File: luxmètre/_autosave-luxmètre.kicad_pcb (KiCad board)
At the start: 2 copper layers, 91.4 x 86.4 mm, 84 parts, among them J1 USB_A, J2 Conn_01x08, J3 Conn_01x01, J4 Conn_01x04, J5 Conn_01x01, J6 Conn_01x01, J7 Conn_01x03, J8 Conn_01x03, SW1 B3S-1000P, U1 ESP32-WROOM-32, U10 MAX1674EUA+T, U11 MCP73831-2-MC, U3 ADC-10-4+, U4 RF-LORA-868-SO, U5 PCA9537DP, U6 FT232HL, U7 ILB1206ER260V, U8 ILB1206ER260V, U9 ILB1206ER260V, Y1 12MHz

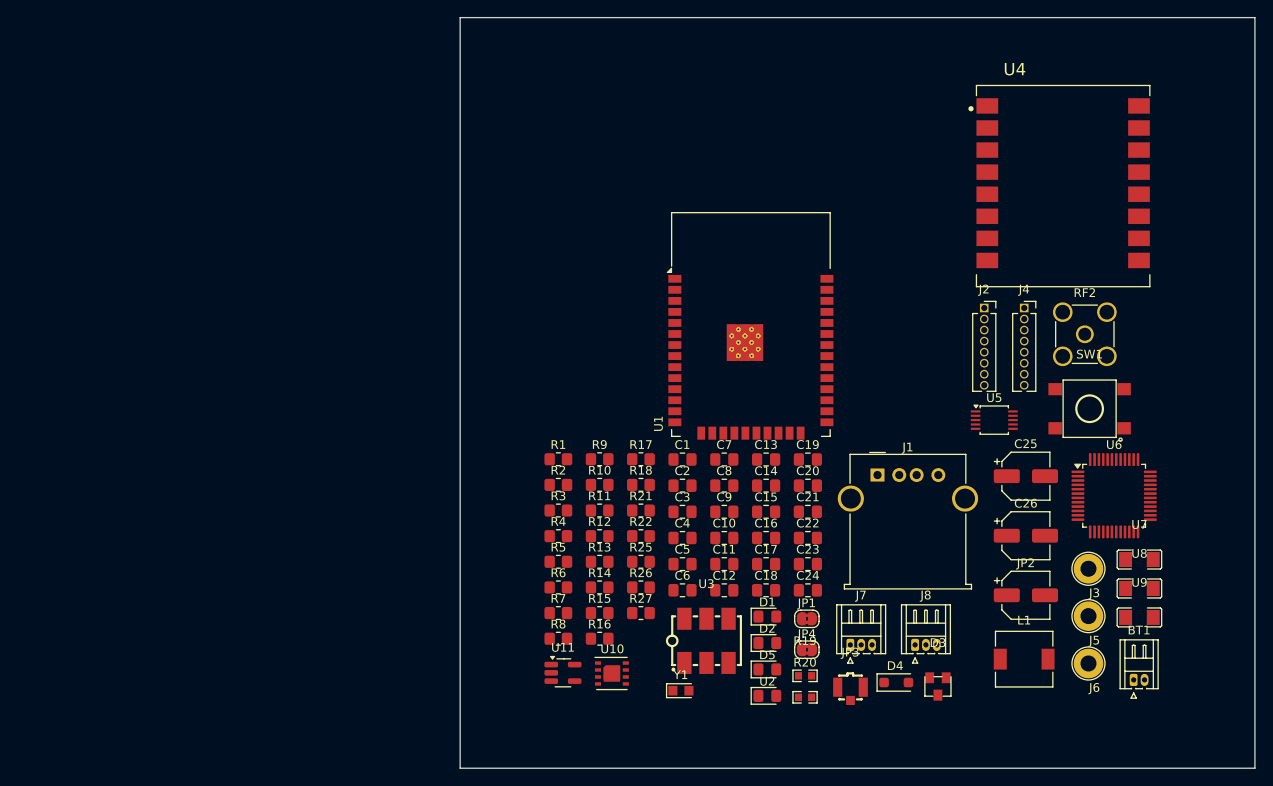
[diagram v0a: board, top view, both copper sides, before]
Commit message: routage computing unit bloc
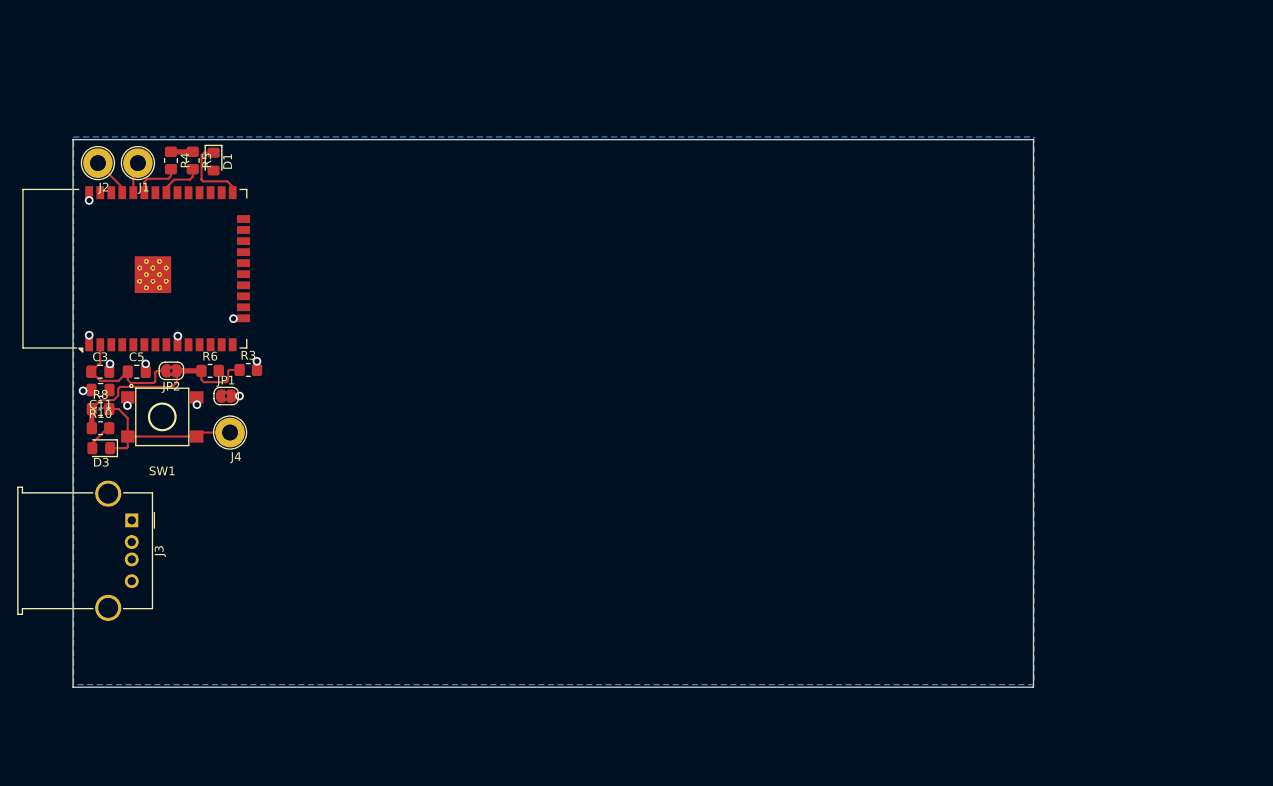
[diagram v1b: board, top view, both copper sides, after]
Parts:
- removed BT1: Battery, Connector_Hirose:Hirose_DF13-02P-1.25DS_1x02_P1.25mm_Horizontal
- removed C1, C10, C13, C14, C15, C16, C2, C23, C24, C7, C8, C9: 100nF, Capacitor_SMD:C_0805_2012Metric_Pad1.18x1.45mm_HandSolder
- removed C12: 3.3uF, Capacitor_SMD:C_0805_2012Metric_Pad1.18x1.45mm_HandSolder
- removed C17, C18, C22, C4, C6: 10uF, Capacitor_SMD:C_0805_2012Metric_Pad1.18x1.45mm_HandSolder
- removed C19, C20, C21: 10nF, Capacitor_SMD:C_0805_2012Metric_Pad1.18x1.45mm_HandSolder
- removed C25, C26: 47uF, Capacitor_SMD:CP_Elec_5x5.4
- removed D2, D5: LED, LED_SMD:LED_0805_2012Metric_Pad1.15x1.40mm_HandSolder
- removed D4: MBR0520LT, Diode_SMD:D_SOD-123F
- removed J5, J6: Conn_01x01, TestPoint:TestPoint_Loop_D2.50mm_Drill1.85mm
- removed J7, J8: Conn_01x03, Connector_Hirose:Hirose_DF13-03P-1.25DS_1x03_P1.25mm_Horizontal
- removed JP3: U.FL-R-SMT-1(80), easyeda2kicad:RF-SMD_FRF05002-JSS103M
- removed JP4: Jumper_2_Open, Jumper:SolderJumper-2_P1.3mm_Bridged2Bar_RoundedPad1.0x1.5mm
- removed L1: 22uH, Inductor_SMD:L_6.3x6.3_H3
- removed R1, R22, R25: 100k, Resistor_SMD:R_0805_2012Metric_Pad1.20x1.40mm_HandSolder
- removed R11, R7: 270R, Resistor_SMD:R_0805_2012Metric_Pad1.20x1.40mm_HandSolder
- removed R12, R9: 68R, Resistor_SMD:R_0805_2012Metric_Pad1.20x1.40mm_HandSolder
- removed R13, R17, R18: 10k, Resistor_SMD:R_0805_2012Metric_Pad1.20x1.40mm_HandSolder
- removed R14, R15: 470R, Resistor_SMD:R_0805_2012Metric_Pad1.20x1.40mm_HandSolder
- removed R16: 47k, Resistor_SMD:R_0805_2012Metric_Pad1.20x1.40mm_HandSolder
- removed R19, R20: V5.5MLA0603NH, easyeda2kicad:R0603
- removed R2: 4k7, Resistor_SMD:R_0805_2012Metric_Pad1.20x1.40mm_HandSolder
- removed R21: 113k, Resistor_SMD:R_0805_2012Metric_Pad1.20x1.40mm_HandSolder
- removed R26: 1.5k, Resistor_SMD:R_0805_2012Metric_Pad1.20x1.40mm_HandSolder
- removed R27: 2k, Resistor_SMD:R_0805_2012Metric_Pad1.20x1.40mm_HandSolder
- removed RF2: HJ-SMA313, Connector_Coaxial:SMA_Amphenol_901-144_Vertical
- removed U1: ESP32-WROOM-32, RF_Module:ESP32-WROOM-32
- removed U10: MAX1674EUA+T, Converter_DCDC:Converter_DCDC_Cyntec_MUN12AD01-SH
- removed U11: MCP73831-2-MC, Package_TO_SOT_SMD:SOT-23-5_HandSoldering
- removed U2: ~, LED_SMD:LED_0805_2012Metric_Pad1.15x1.40mm_HandSolder
- removed U3: ADC-10-4+, My_symbols:XFMR-SMD_6P-L7.9-W5.6-P2.54-LS7.0-BL
- removed U5: PCA9537DP, Package_SO:TSSOP-10_3x3mm_P0.5mm
- removed U6: FT232HL, Package_QFP:LQFP-48_7x7mm_P0.5mm
- removed U7, U8, U9: ILB1206ER260V, easyeda2kicad:L1206
- removed Y1: 12MHz, Crystal:Crystal_SMD_2012-2Pin_2.0x1.2mm_HandSoldering
- C5: value 100nF -> 10uF
- D3: value PGB102ST23WR -> LED; footprint easyeda2kicad:SOT-23_L3.0-W2.2-P0.95-LS2.2-TR -> LED_SMD:LED_0805_2012Metric_Pad1.15x1.40mm_HandSolder
- J1: value USB_A -> Conn_01x01; footprint Connector_USB:USB_A_Molex_67643_Horizontal -> TestPoint:TestPoint_Loop_D2.50mm_Drill1.85mm
- J2: value Conn_01x08 -> Conn_01x01; footprint Connector_PinSocket_1.27mm:PinSocket_1x08_P1.27mm_Vertical -> TestPoint:TestPoint_Loop_D2.50mm_Drill1.85mm
- J3: value Conn_01x01 -> USB_A; footprint TestPoint:TestPoint_Loop_D2.50mm_Drill1.85mm -> Connector_USB:USB_A_Molex_67643_Horizontal
- J4: value Conn_01x04 -> Conn_01x01; footprint Connector_PinSocket_1.27mm:PinSocket_1x08_P1.27mm_Vertical -> TestPoint:TestPoint_Loop_D2.50mm_Drill1.85mm
- JP2: footprint Capacitor_SMD:CP_Elec_5x5.4 -> Jumper:SolderJumper-2_P1.3mm_Bridged2Bar_RoundedPad1.0x1.5mm
- R10: value 68R -> 470R
- R3: value 4k7 -> 10k
- R4: value 10k -> 4k7
- R5: value 100k -> 4k7
- R6: value R -> 470R
- R8: value 68R -> 10k
- U4: value RF-LORA-868-SO -> ESP32-WROOM-32; footprint My_symbols:XCVR_RF-LORA-868-SO -> RF_Module:ESP32-WROOM-32
- moved J3 110.2 mm to (56.2, 93.4), turned to -90 degrees
- moved SW1 106.7 mm to (59.7, 81.5), turned to 180 degrees
- moved U4 104.2 mm to (59.5, 64.5), turned to 90 degrees
- moved J2 103.3 mm to (52.3, 52.3)
- moved JP2 101.6 mm to (60.8, 76.2), turned to 180 degrees
- moved D3 100.1 mm to (52.7, 85.1), turned to 180 degrees
- moved J4 92.5 mm to (67.5, 83.3)
- moved J1 92.3 mm to (56.9, 52.3)
- moved D1 82.5 mm to (65.6, 52.1), turned to -90 degrees
- moved C11 74.5 mm to (52.6, 78.4), turned to 180 degrees
- moved JP1 71.6 mm to (67.1, 79.1)
- moved C3 68.9 mm to (52.6, 76.3)
- moved C5 66.6 mm to (56.8, 76.3)
- moved R5 62.5 mm to (63.2, 52.0), turned to -90 degrees
- moved R4 62.1 mm to (60.7, 52.0), turned to -90 degrees
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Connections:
- C11 pad 1: Net-(U6-VCCA) -> /RST
- C3 pad 1: +3.3V -> Net-(JP2-B)
- C5 pad 1: Net-(JP4-B) -> Net-(JP2-B)
- D1 pad 1: //RST -> /BOOT
- D3 pad 1: /dp -> /RST
- D3 pad 2: /dm -> Net-(D3-A)
- J1 pad 1: /5V_usb -> /RXD
- J2 pad 1: /DIO0 -> /TXD
- J3 pad 1: //RST -> /5V_usb
- J4 pad 1: /RST_L -> /RST
- R10 pad 1: GND -> +3.3V
- R10 pad 2: Net-(R10-Pad2) -> Net-(D3-A)
- R3 pad 2: /SCL -> GND
- R4 pad 2: GND -> /SCL
- R5 pad 1: GND -> +3.3V
- R5 pad 2: /TX_SW -> /SDA
- R6 pad 1: GND -> +3.3V
- R6 pad 2: Net-(U3-TERM) -> Net-(D1-A)
- R8 pad 1: GND -> +3.3V
- R8 pad 2: /C -> /RST
- SW1 pad 3: //RST -> /RST
- SW1 pad 4: //RST -> /RST
- U4 pad 1: /ANT -> GND
- U4 pad 10: /DIO4 -> unconnected-(U4-IO25-Pad10)
- U4 pad 11: /DIO3 -> unconnected-(U4-IO26-Pad11)
- U4 pad 12: /RST_L -> unconnected-(U4-IO27-Pad12)
- U4 pad 14: /MOSI_L -> /MISO_L
- U4 pad 15: /MISO_L -> GND
- U4 pad 16: //SEL -> /MOSI_L
- U4 pad 2: GND -> Net-(JP2-B)
- U4 pad 3: Net-(JP2-B) -> /RST
- U4 pad 4: /RX_SW -> unconnected-(U4-SENSOR_VP-Pad4)
- U4 pad 5: /TX_SW -> unconnected-(U4-SENSOR_VN-Pad5)
- U4 pad 6: /DIO0 -> unconnected-(U4-IO34-Pad6)
- U4 pad 7: /DIO1 -> unconnected-(U4-IO35-Pad7)
- U4 pad 8: /DIO2 -> unconnected-(U4-IO32-Pad8)
- U4 pad 9: /DIO5 -> GND
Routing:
- net +3.3V: track 0.00 -> 27.1 mm
- net /RST: track 0.00 -> 19.9 mm
- net Net-(JP2-B): track 0.00 -> 15.2 mm
- net GND: track 0.00 -> 10.8 mm, vias 0 -> 11
- net /BOOT: track 0.00 -> 8.95 mm
- net /SCL: track 0.00 -> 5.37 mm
- net /SDA: track 0.00 -> 5.01 mm
- net /TXD: track 0.00 -> 4.56 mm
- net /RXD: track 0.00 -> 3.62 mm
- net Net-(D3-A): track 0.00 -> 3.23 mm
- added copper zone on B.Cu, net GND
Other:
- board size 91.4 x 86.4 mm -> 110.5 x 63 mm
- copper layers 2 -> 4

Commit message: pcb
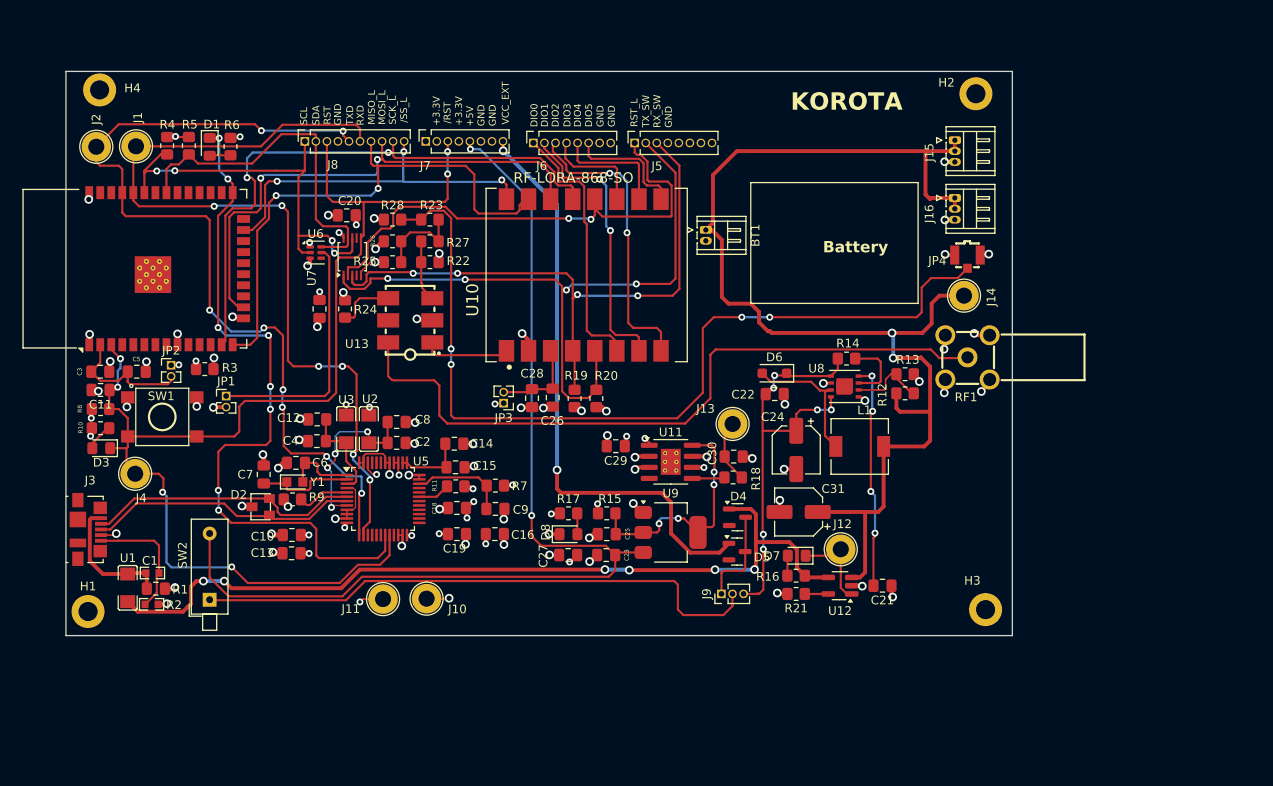
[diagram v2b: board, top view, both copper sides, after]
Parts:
- added BT1: Battery, Connector_Hirose:Hirose_DF13-02P-1.25DS_1x02_P1.25mm_Horizontal, F.Cu at (122.2, 60.0)
- added C1: 10uF, Capacitor_SMD:C_0805_2012Metric_Pad1.18x1.45mm_HandSolder, F.Cu at (59.0, 101.3)
- added C10: 100nF, Capacitor_SMD:C_0805_2012Metric_Pad1.18x1.45mm_HandSolder, F.Cu at (74.6, 95.1)
- added C12: 100nF, Capacitor_SMD:C_0805_2012Metric_Pad1.18x1.45mm_HandSolder, F.Cu at (77.5, 81.8)
- added C13: 100nF, Capacitor_SMD:C_0805_2012Metric_Pad1.18x1.45mm_HandSolder, F.Cu at (74.6, 97.2)
- added C14: 3.3uF, Capacitor_SMD:C_0805_2012Metric_Pad1.18x1.45mm_HandSolder, F.Cu at (93.3, 84.6)
- added C15: 100nF, Capacitor_SMD:C_0805_2012Metric_Pad1.18x1.45mm_HandSolder, F.Cu at (93.4, 87.3)
- added C16: 100nF, Capacitor_SMD:C_0805_2012Metric_Pad1.18x1.45mm_HandSolder, F.Cu at (98.0, 95.0)
- added C17: 100nF, Capacitor_SMD:C_0805_2012Metric_Pad1.18x1.45mm_HandSolder, F.Cu at (77.8, 69.1)
- added C18: 100nF, Capacitor_SMD:C_0805_2012Metric_Pad1.18x1.45mm_HandSolder, F.Cu at (93.6, 92.0)
- added C19: 100nF, Capacitor_SMD:C_0805_2012Metric_Pad1.18x1.45mm_HandSolder, F.Cu at (93.6, 95.0)
- added C2: 10uF, Capacitor_SMD:C_0805_2012Metric_Pad1.18x1.45mm_HandSolder, F.Cu at (86.7, 84.5)
- added C20: 100nF, Capacitor_SMD:C_0805_2012Metric_Pad1.18x1.45mm_HandSolder, F.Cu at (80.9, 58.3)
- added C21: 100nF, Capacitor_SMD:C_0805_2012Metric_Pad1.18x1.45mm_HandSolder, F.Cu at (142.6, 100.9)
- added C22: 100nF, Capacitor_SMD:C_0805_2012Metric_Pad1.18x1.45mm_HandSolder, F.Cu at (130.2, 78.9)
- added C23: 10uF, Capacitor_SMD:C_0805_2012Metric_Pad1.18x1.45mm_HandSolder, F.Cu at (110.8, 97.4)
- added C24: 47uF, Capacitor_SMD:CP_Elec_5x5.4, F.Cu at (132.7, 85.3)
- added C25: 10uF, Capacitor_SMD:C_0805_2012Metric_Pad1.18x1.45mm_HandSolder, F.Cu at (110.8, 95.0)
- added C26: 100nF, Capacitor_SMD:C_0805_2012Metric_Pad1.18x1.45mm_HandSolder, F.Cu at (104.6, 79.3)
- added C27: 100nF, Capacitor_SMD:C_0805_2012Metric_Pad1.18x1.45mm_HandSolder, F.Cu at (106.4, 97.4)
- added C28: 10uF, Capacitor_SMD:C_0805_2012Metric_Pad1.18x1.45mm_HandSolder, F.Cu at (102.2, 79.3)
- added C29: 100nF, Capacitor_SMD:C_0805_2012Metric_Pad1.18x1.45mm_HandSolder, F.Cu at (111.9, 84.9)
- added C30: 10nF, Capacitor_SMD:C_0805_2012Metric_Pad1.18x1.45mm_HandSolder, F.Cu at (125.4, 86.1)
- added C31: 47uF, Capacitor_SMD:CP_Elec_5x5.4, F.Cu at (132.9, 92.4)
- added C4: 10uF, Capacitor_SMD:C_0805_2012Metric_Pad1.18x1.45mm_HandSolder, F.Cu at (77.5, 84.3)
- added C6: 10nF, Capacitor_SMD:C_0805_2012Metric_Pad1.18x1.45mm_HandSolder, F.Cu at (75.1, 86.8)
- added C7: 10nF, Capacitor_SMD:C_0805_2012Metric_Pad1.18x1.45mm_HandSolder, F.Cu at (71.4, 88.1)
- added C8: 100nF, Capacitor_SMD:C_0805_2012Metric_Pad1.18x1.45mm_HandSolder, F.Cu at (86.7, 82.1)
- added C9: 10nF, Capacitor_SMD:C_0805_2012Metric_Pad1.18x1.45mm_HandSolder, F.Cu at (98.0, 92.1)
- added D2: PGB102ST23WR, easyeda2kicad:SOT-23_L3.0-W2.2-P0.95-LS2.2-TR, F.Cu at (71.0, 91.8)
- added D4: BAT54C, Package_TO_SOT_SMD:SOT-23, F.Cu at (125.9, 93.0)
- added D5: BAT54C, Package_TO_SOT_SMD:SOT-23, F.Cu at (125.8, 97.0)
- added D6: MBR0520LT, Diode_SMD:D_SOD-123F, F.Cu at (130.1, 76.5)
- added D7: LED, LED_SMD:LED_0805_2012Metric_Pad1.15x1.40mm_HandSolder, F.Cu at (132.7, 97.5)
- added D8: LED, LED_SMD:LED_0805_2012Metric_Pad1.15x1.40mm_HandSolder, F.Cu at (106.4, 95.0)
- added H1: MountingHole, MountingHole:MountingHole_2.2mm_M2_DIN965_Pad, F.Cu at (51.2, 103.9)
- added H2: MountingHole, MountingHole:MountingHole_2.2mm_M2_DIN965_Pad, F.Cu at (153.3, 44.3)
- added H3: MountingHole, MountingHole:MountingHole_2.2mm_M2_DIN965_Pad, F.Cu at (154.4, 103.7)
- added H4: MountingHole, MountingHole:MountingHole_2.2mm_M2_DIN965_Pad, F.Cu at (52.5, 43.9)
- added J10: Conn_01x01, TestPoint:TestPoint_Loop_D2.50mm_Drill1.85mm, F.Cu at (90.1, 102.4)
- added J11: Conn_01x01, TestPoint:TestPoint_Loop_D2.50mm_Drill1.85mm, F.Cu at (85.1, 102.5)
- added J12: Conn_01x01, TestPoint:TestPoint_Loop_D2.50mm_Drill1.85mm, F.Cu at (137.8, 96.7)
- added J13: Conn_01x01, TestPoint:TestPoint_Loop_D2.50mm_Drill1.85mm, F.Cu at (125.3, 82.3)
- added J14: Conn_01x01, TestPoint:TestPoint_Loop_D2.50mm_Drill1.85mm, F.Cu at (151.9, 67.5)
- added J15: Conn_01x03, Connector_Hirose:Hirose_DF13-03P-1.25DS_1x03_P1.25mm_Horizontal, F.Cu at (150.9, 49.7)
- added J16: Conn_01x03, Connector_Hirose:Hirose_DF13-03P-1.25DS_1x03_P1.25mm_Horizontal, F.Cu at (150.9, 56.3)
- added J5: Conn_01x04, Connector_PinSocket_1.27mm:PinSocket_1x08_P1.27mm_Vertical, F.Cu at (114.1, 50.0)
- added J6: Conn_01x08, Connector_PinSocket_1.27mm:PinSocket_1x08_P1.27mm_Vertical, F.Cu at (102.4, 50.0)
- added J7: Conn_01x08, Connector_PinSocket_1.27mm:PinSocket_1x08_P1.27mm_Vertical, F.Cu at (90.0, 49.8)
- added J8: Conn_01x10, Connector_PinSocket_1.27mm:PinSocket_1x10_P1.27mm_Vertical, F.Cu at (76.1, 49.8)
- added J9: Conn_01x03, Connector_PinHeader_1.27mm:PinHeader_1x03_P1.27mm_Vertical, F.Cu at (124.0, 101.9)
- added JP3: Jumper_2_Open, Connector_PinHeader_1.27mm:PinHeader_1x02_P1.27mm_Vertical, F.Cu at (99.0, 79.9)
- added JP4: U.FL-R-SMT-1(80), easyeda2kicad:RF-SMD_FRF05002-JSS103M, F.Cu at (152.3, 63.6)
- added L1: 22uH, Inductor_SMD:L_6.3x6.3_H3, F.Cu at (139.9, 84.9)
- added R1: V5.5MLA0603NH, easyeda2kicad:R0603, F.Cu at (58.6, 99.5)
- added R11: 47k, Resistor_SMD:R_0805_2012Metric_Pad1.20x1.40mm_HandSolder, F.Cu at (93.5, 89.5)
- added R12: 113k, Resistor_SMD:R_0805_2012Metric_Pad1.20x1.40mm_HandSolder, F.Cu at (145.2, 78.8)
- added R13: 100k, Resistor_SMD:R_0805_2012Metric_Pad1.20x1.40mm_HandSolder, F.Cu at (145.2, 76.6)
- added R14: 100k, Resistor_SMD:R_0805_2012Metric_Pad1.20x1.40mm_HandSolder, F.Cu at (138.4, 74.8)
- added R15: 0R1, Resistor_SMD:R_0805_2012Metric_Pad1.20x1.40mm_HandSolder, F.Cu at (110.8, 92.6)
- added R16: 1.5k, Resistor_SMD:R_0805_2012Metric_Pad1.20x1.40mm_HandSolder, F.Cu at (132.6, 99.8)
- added R17: 330R, Resistor_SMD:R_0805_2012Metric_Pad1.20x1.40mm_HandSolder, F.Cu at (106.4, 92.6)
- added R18: 330R, Resistor_SMD:R_0805_2012Metric_Pad1.20x1.40mm_HandSolder, F.Cu at (125.4, 88.5)
- added R19: 100k, Resistor_SMD:R_0805_2012Metric_Pad1.20x1.40mm_HandSolder, F.Cu at (107.2, 79.4)
- added R2: V5.5MLA0603NH, easyeda2kicad:R0603, F.Cu at (58.5, 103.1)
- added R20: 100k, Resistor_SMD:R_0805_2012Metric_Pad1.20x1.40mm_HandSolder, F.Cu at (109.7, 79.4)
- added R21: 2k, Resistor_SMD:R_0805_2012Metric_Pad1.20x1.40mm_HandSolder, F.Cu at (132.6, 101.9)
- added R22: 68R, Resistor_SMD:R_0805_2012Metric_Pad1.20x1.40mm_HandSolder, F.Cu at (90.5, 63.7)
- added R23: 270R, Resistor_SMD:R_0805_2012Metric_Pad1.20x1.40mm_HandSolder, F.Cu at (90.5, 61.3)
- added R24: R, Resistor_SMD:R_0805_2012Metric_Pad1.20x1.40mm_HandSolder, F.Cu at (80.7, 69.1)
- added R25: 68R, Resistor_SMD:R_0805_2012Metric_Pad1.20x1.40mm_HandSolder, F.Cu at (86.2, 63.7)
- added R26: 68R, Resistor_SMD:R_0805_2012Metric_Pad1.20x1.40mm_HandSolder, F.Cu at (86.2, 61.3)
- added R27: 270R, Resistor_SMD:R_0805_2012Metric_Pad1.20x1.40mm_HandSolder, F.Cu at (90.5, 58.8)
- added R28: 68R, Resistor_SMD:R_0805_2012Metric_Pad1.20x1.40mm_HandSolder, F.Cu at (86.2, 58.8)
- added R7: 10k, Resistor_SMD:R_0805_2012Metric_Pad1.20x1.40mm_HandSolder, F.Cu at (98.0, 89.4)
- added R9: 10k, Resistor_SMD:R_0805_2012Metric_Pad1.20x1.40mm_HandSolder, F.Cu at (74.7, 91.0)
- added RF1: HJ-SMA313, easyeda2kicad:SMA-TH_HJ-2LC15SF048, F.Cu at (152.3, 74.7)
- added SW2: SW_DIP_x01, Button_Switch_THT:SW_DIP_SPSTx01_Piano_10.8x4.1mm_W7.62mm_P2.54mm, F.Cu at (65.2, 102.5)
- added U1: ILB1206ER260V, easyeda2kicad:L1206, F.Cu at (55.7, 101.2)
- added U10: RF-LORA-868-SO, My_symbols:XCVR_RF-LORA-868-SO, F.Cu at (108.5, 65.2)
- added U11: AD8418, Package_SO:SOIC-8-1EP_3.9x4.9mm_P1.27mm_EP2.29x3mm_ThermalVias, F.Cu at (118.2, 86.7)
- added U12: MCP73831-2-MC, Package_TO_SOT_SMD:SOT-23-5_HandSoldering, F.Cu at (137.7, 100.9)
- added U13: ADC-10-4+, My_symbols:XFMR-SMD_6P-L7.9-W5.6-P2.54-LS7.0-BL, F.Cu at (88.2, 70.4)
- added U2: ILB1206ER260V, easyeda2kicad:L1206, F.Cu at (83.5, 82.9)
- added U3: ILB1206ER260V, easyeda2kicad:L1206, F.Cu at (80.9, 82.9)
- added U5: FT232HL, Package_QFP:LQFP-48_7x7mm_P0.5mm, F.Cu at (85.1, 90.9)
- added U6: ~, OptoDevice:AMS_TSL25911FN, F.Cu at (77.4, 62.6)
- added U7: PCA9537DP, Package_SO:TSSOP-10_3x3mm_P0.5mm, F.Cu at (81.6, 63.1)
- added U8: MAX1674EUA+T, Converter_DCDC:Converter_DCDC_Cyntec_MUN12AD01-SH, F.Cu at (138.2, 78.0)
- added U9: LM1117MP-3.3, Package_TO_SOT_SMD:SOT-223-3_TabPin2, F.Cu at (118.2, 94.8)
- added Y1: 12MHz, Crystal:Crystal_SMD_2012-2Pin_2.0x1.2mm_HandSoldering, F.Cu at (75.0, 89.0)
- J3: footprint Connector_USB:USB_A_Molex_67643_Horizontal -> Connector_USB:USB_Micro-B_Molex_47346-0001
- JP1, JP2: footprint Jumper:SolderJumper-2_P1.3mm_Bridged2Bar_RoundedPad1.0x1.5mm -> Connector_PinHeader_1.27mm:PinHeader_1x02_P1.27mm_Vertical
- moved R6 25.9 mm to (67.6, 50.4), turned to -90 degrees
- moved J4 11.9 mm to (56.6, 88.0)
- moved J3 5.11 mm to (51.2, 94.5)
- moved R3 5.01 mm to (64.6, 76.0)
- moved J1 1.94 mm to (56.7, 50.4)
- moved J2 1.89 mm to (52.1, 50.4)
- moved D1 1.76 mm to (65.2, 50.4)
- moved R4 1.76 mm to (60.3, 50.3)
- moved R5 1.76 mm to (62.8, 50.3)
- moved JP2 0.64 mm to (60.7, 75.6), turned to 0 degrees
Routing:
- net V_BAT: track 0.00 -> 140.2 mm, vias 0 -> 2
- net /RST: track 19.9 -> 143.8 mm, vias 0 -> 6
- net +5V: track 0.00 -> 118.5 mm, vias 0 -> 2
- net Net-(JP4-SIG): track 0.00 -> 101.9 mm, vias 0 -> 4
- net GND: track 10.8 -> 110.7 mm, vias 11 -> 76
- net /TXD: track 4.56 -> 102.2 mm, vias 0 -> 8
- net VCC_USB: track 0.00 -> 97.6 mm, vias 0 -> 6
- net /RXD: track 3.62 -> 98.6 mm, vias 0 -> 6
- net Net-(U13-OUTPUT): track 0.00 -> 81.7 mm
- net /TX_SW: track 0.00 -> 79.3 mm, vias 0 -> 4
- net /BOOT: track 8.95 -> 81.3 mm, vias 0 -> 8
- net /RX_SW: track 0.00 -> 71.2 mm, vias 0 -> 4
- net /SCK_L: track 0.00 -> 67.9 mm, vias 0 -> 2
- net VCC_EXT: track 0.00 -> 67.9 mm, vias 0 -> 2
- net Net-(J9-Pin_2): track 0.00 -> 66.2 mm
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- added copper zone on In2.Cu, net +3.3V
- added copper zone on In1.Cu, net GND
- removed copper zone on B.Cu, net GND
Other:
- board size 110.5 x 63 mm -> 108.9 x 64.9 mm
- board text added: "+3.3V"
- board text added: "+5V"
- board text added: "/RST"
- board text added: "/SS_L"
- board text added: "Battery"
- board text added: "DIO0"
- board text added: "DIO1"
- board text added: "DIO2"
- board text added: "DIO3"
- board text added: "DIO4"
- board text added: "DIO5"
- board text added: "GND"
- board text added: "KOROTA"
- board text added: "MISO_L"
- board text added: "MOSI_L"
- board text added: "RF-LORA-868-SO"
- board text added: "RST"
- board text added: "RST_L"
- board text added: "RXD"
- board text added: "RX_SW"
- board text added: "SCK_L"
- board text added: "SCL"
- board text added: "SDA"
- board text added: "TXD"
- board text added: "TX_SW"
- board text added: "VCC_EXT"

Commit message: pcb
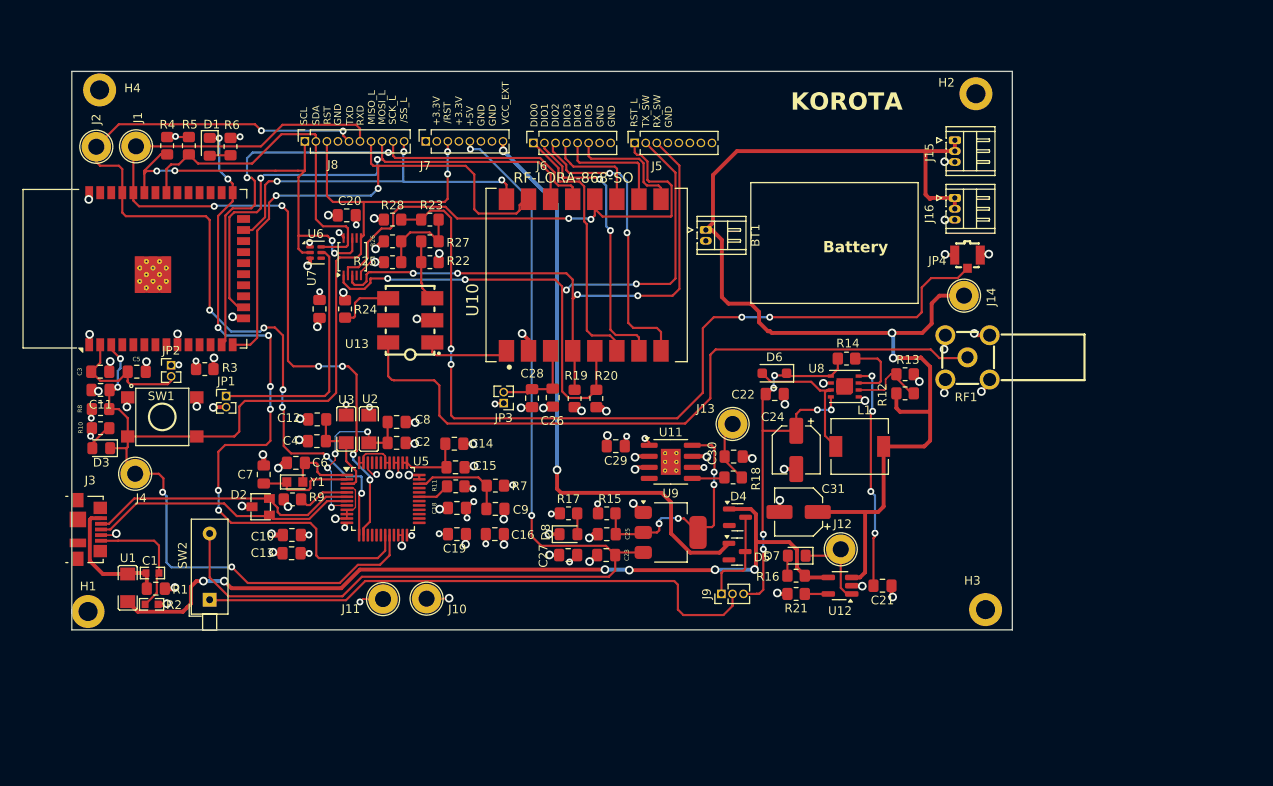
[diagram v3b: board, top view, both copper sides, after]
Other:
- board size 108.9 x 64.9 mm -> 108.2 x 64.2 mm
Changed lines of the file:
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@@
 			(outputformat 1)
 			(mirror no)
-			(drillshape 1)
+			(drillshape 0)
 			(scaleselection 1)
 			(outputdirectory "")
@@
 	)
 	(gr_rect
-		(start 48.63 41.75)
-		(end 157.51 106.66)
+		(start 49.3 41.75)
+		(end 157.51 106)
 		(stroke
 			(width 0.05)
@@
 		(polygon
 			(pts
-				(xy 49.52 42.09) (xy 158.12 41.9) (xy 157.31 106.38) (xy 48.68 106.79)
+				(xy 48.42 41.69) (xy 157.02 41.5) (xy 158.51 105.98) (xy 49.88 106.39)
 			)
 		)
@@
 		(polygon
 			(pts
-				(xy 49.1 42.12) (xy 158.13 41.25) (xy 157.08 106.27) (xy 48.67 107.15)
+				(xy 49 42.12) (xy 158.03 41.25) (xy 157.78 105.67) (xy 49.37 106.55)
 			)
 		)
